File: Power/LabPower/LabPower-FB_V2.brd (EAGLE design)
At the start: 27.3 x 38.1 mm, 25 parts, among them IC1 INA168, IC2 LD117ASTR, U1 TSV621ILT

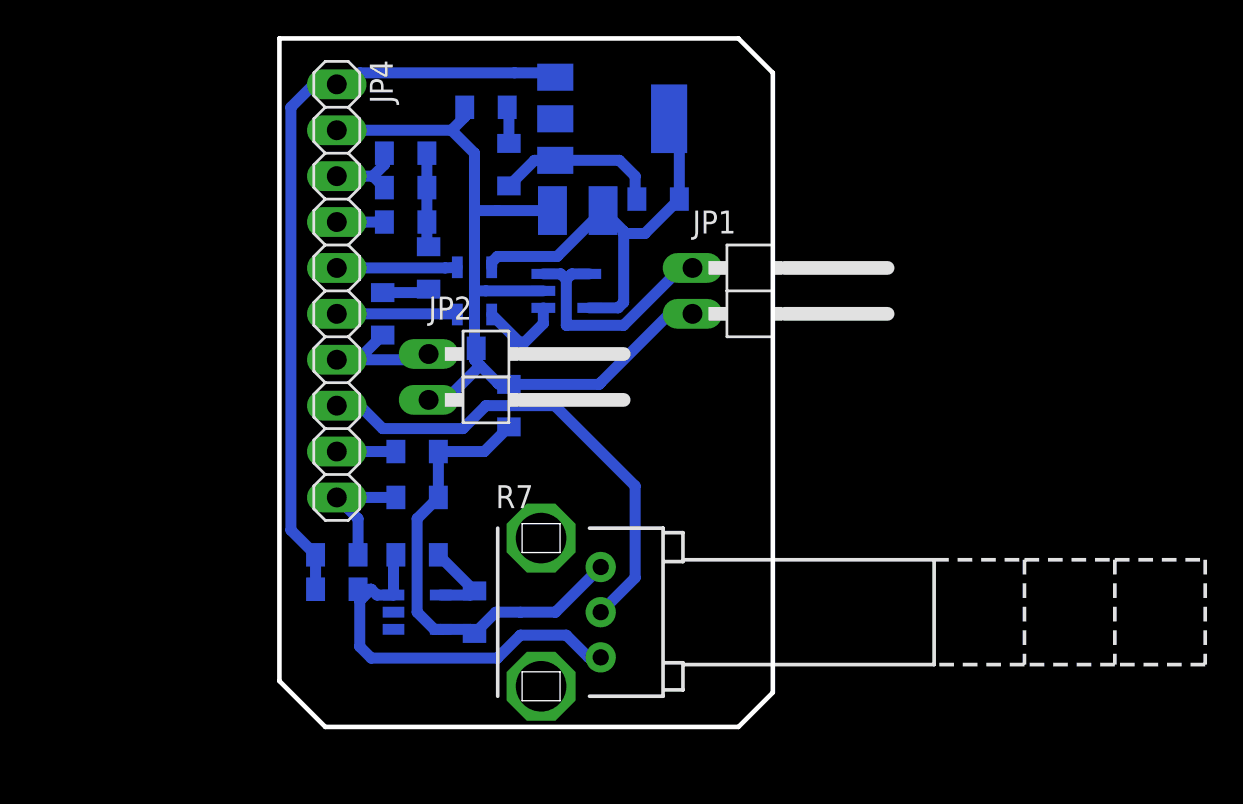
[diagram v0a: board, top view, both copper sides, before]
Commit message: Опять всё неправильно сделал
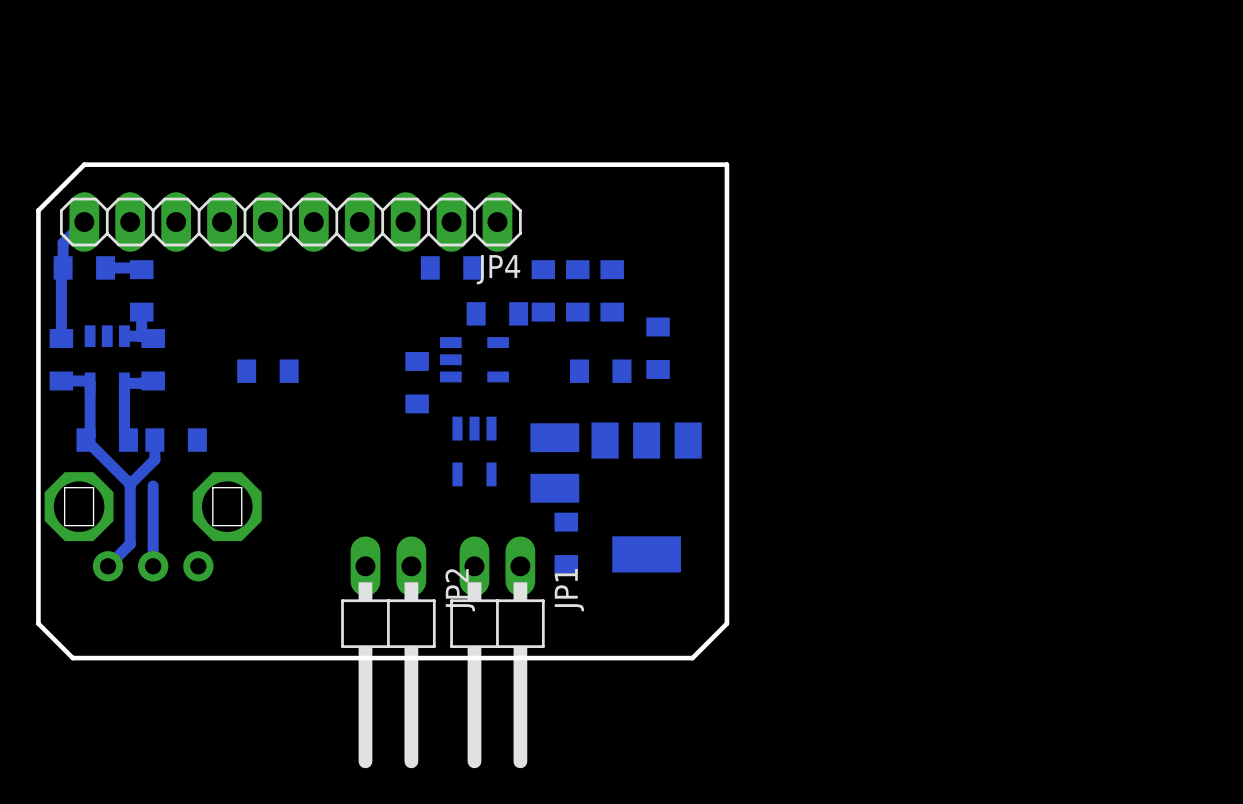
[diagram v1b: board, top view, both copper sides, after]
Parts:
- moved R7 24.9 mm to (-8.26, -27.9), flipped to the bottom, turned to 270 degrees
- moved JP1 24.0 mm to (10.8, -31.8), turned to 180 degrees
- moved R5 22.4 mm to (-10.8, -21.0), turned to 180 degrees
- moved U$1 22.4 mm to (-10.8, -17.8), turned to 180 degrees
- moved R8 21.1 mm to (-12.1, -11.4), turned to 180 degrees
- moved R9 21.1 mm to (-13.3, -16.5), turned to 90 degrees
- moved IC2 21.0 mm to (19.1, -24.1), turned to 180 degrees
- moved R4 19.7 mm to (-8.89, -12.7), turned to 90 degrees
- moved R12 19.7 mm to (14.6, -26.7), turned to 270 degrees
- moved R17 18.5 mm to (-6.99, -21.0), turned to 180 degrees
- moved R6 18.2 mm to (-8.26, -16.5), turned to 90 degrees
- moved R14 16.4 mm to (19.7, -15.9), turned to 270 degrees
- moved JP2 15.5 mm to (4.76, -31.8), turned to 180 degrees
- moved C1 14.0 mm to (14.0, -22.2), turned to 90 degrees
- moved R1 13.7 mm to (17.1, -12.7), turned to 90 degrees
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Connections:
- new net N$11: IC1.5, U1.5
- net N$9: no longer IC1.5, U1.5
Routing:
- net GND: track 47.5 -> 0.00 mm
- net +12V: track 43.1 -> 2.04 mm
- net N$9: track 24.1 -> 0.00 mm
- net -V-FB: track 27.2 -> 4.45 mm
- net N$1: track 22.4 -> 2.98 mm
- net N$7: track 13.6 -> 0.00 mm
- net N$10: track 26.0 -> 16.4 mm
- net N$6: track 9.24 -> 0.00 mm
- net +V-FB: track 7.68 -> 0.00 mm
- net C-IN+: track 6.68 -> 0.00 mm
- net C-IN-: track 6.67 -> 0.00 mm
- net N$8: track 5.29 -> 0.00 mm
- net N$3: track 5.21 -> 0.00 mm
- net V-IN+: track 4.43 -> 0.00 mm
- net +I-FB: track 3.27 -> 0.00 mm
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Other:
- board size 27.3 x 38.1 mm -> 38.1 x 27.3 mm
